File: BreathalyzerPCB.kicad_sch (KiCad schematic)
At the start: 12 parts, among them SW101 SW_SPST, U101 MAX6105, U102 ABX00030, U103 SEN-08880

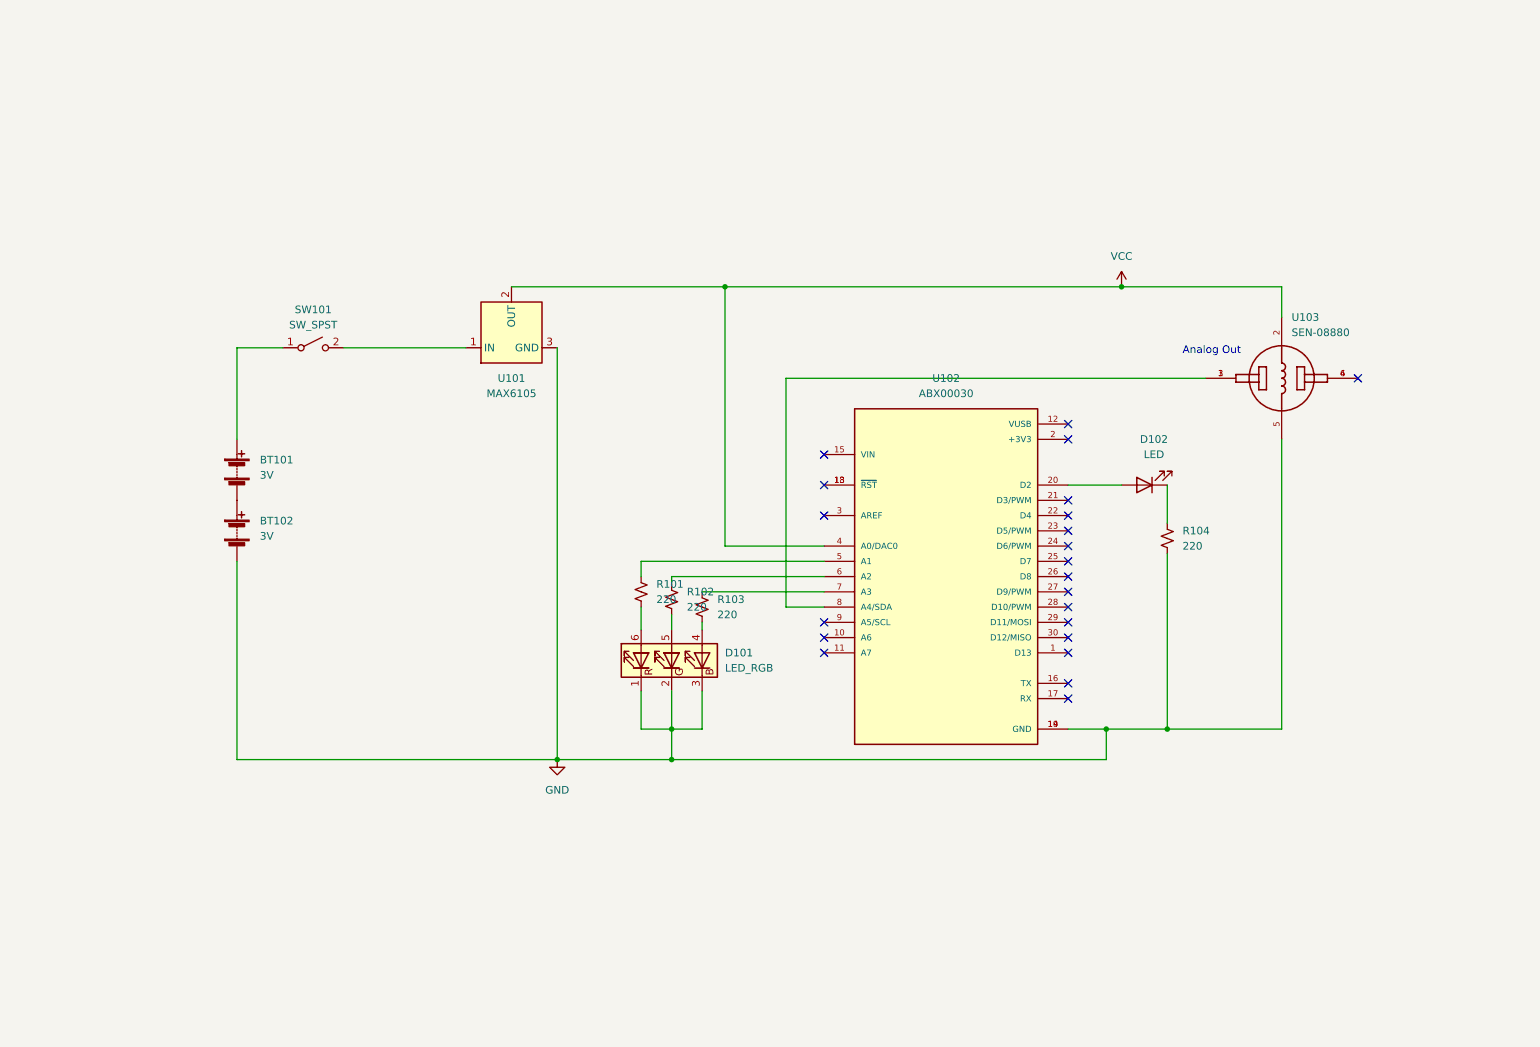
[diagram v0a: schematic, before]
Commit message: v2.1.0
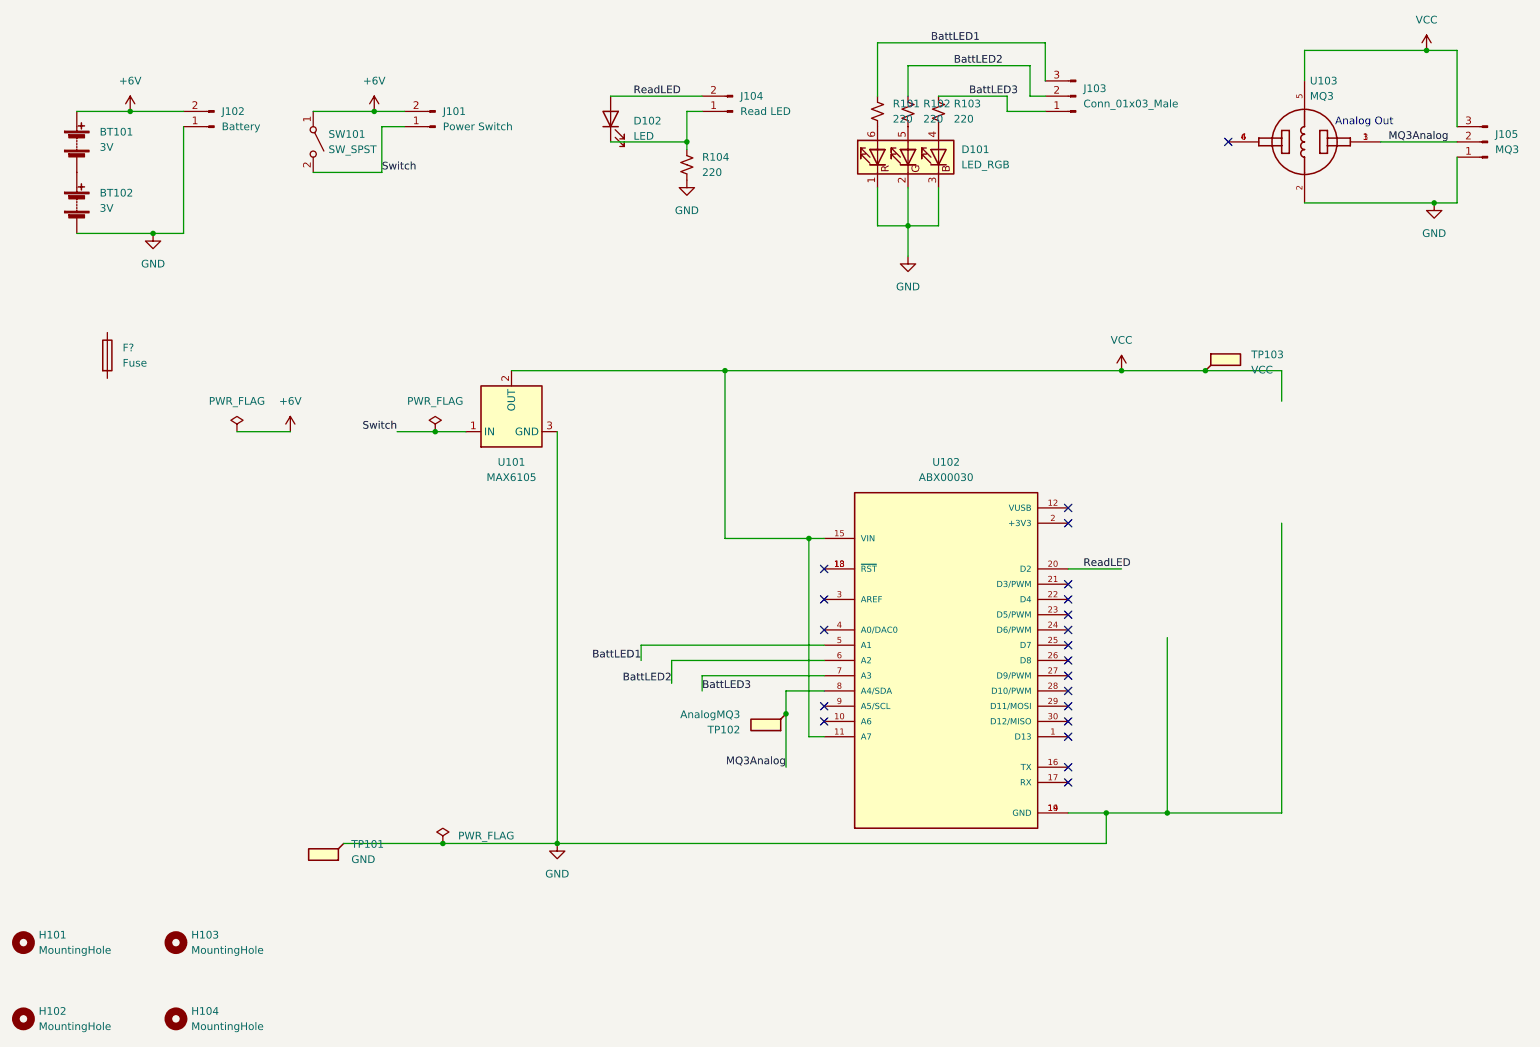
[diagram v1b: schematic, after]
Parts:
- added F?: Fuse, symbol Device:Fuse
- added H101, H102, H103, H104: MountingHole, MountingHole:MountingHole_3.2mm_M3, symbol Mechanical:MountingHole
- added J101: Power Switch, Connector_PinHeader_2.54mm:PinHeader_1x02_P2.54mm_Vertical, symbol Connector:Conn_01x02_Male
- added J102: Battery, Connector_PinHeader_2.54mm:PinHeader_1x02_P2.54mm_Vertical, symbol Connector:Conn_01x02_Male
- added J103: Conn_01x03_Male, Connector_PinHeader_2.54mm:PinHeader_1x03_P2.54mm_Vertical, symbol Connector:Conn_01x03_Male
- added J104: Read LED, Connector_PinHeader_2.54mm:PinHeader_1x02_P2.54mm_Vertical, symbol Connector:Conn_01x02_Male
- added J105: MQ3, Connector_PinHeader_2.54mm:PinHeader_1x03_P2.54mm_Vertical, symbol Connector:Conn_01x03_Male
- added TP101: GND, TestPoint:TestPoint_Pad_D4.0mm, symbol Connector:TestPoint_Flag
- added TP102: AnalogMQ3, TestPoint:TestPoint_Pad_D4.0mm, symbol Connector:TestPoint_Flag
- added TP103: VCC, TestPoint:TestPoint_Pad_D4.0mm, symbol Connector:TestPoint_Flag
- R101, R102, R103, R104: footprint (none) -> Resistor_THT:R_Axial_DIN0309_L9.0mm_D3.2mm_P12.70mm_Horizontal
- U102: footprint MODULE_ABX00030 -> Connector_PinSocket_2.54mm:PinSocket_2x14_P2.54mm_Vertical
- U103: value SEN-08880 -> MQ3
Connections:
- net GND: now also U103.2, J102.1 (Pin_1), J105.1 (Pin_1), TP101.1; no longer U103.5
- net VCC: now also U102.11 (A7), U102.15 (VIN), U103.5, J105.3 (Pin_3), TP103.1; no longer U102.4 (A0/DAC0), U103.2
- net at D102.1 (K), R104.1: now also J104.1 (Pin_1)
- net ReadLED: now reaches D102.2 (A), U102.20 (D2)
- net ReadLED: now also J104.2 (Pin_2)
- net Switch: now reaches SW101.2 (B), U101.1 (IN)
- net Switch: now also J101.1 (Pin_1)
- net +6V: now reaches BT101.1 (+), SW101.1 (A)
- net +6V: now also J101.2 (Pin_2), J102.2 (Pin_2)
- net BattLED1: now reaches R101.1, U102.5 (A1)
- net BattLED1: now also J103.3 (Pin_3)
- net BattLED2: now reaches R102.1, U102.6 (A2)
- net BattLED2: now also J103.2 (Pin_2)
- net BattLED3: now reaches R103.1, U102.7 (A3)
- net BattLED3: now also J103.1 (Pin_1)
- net MQ3Analog: now reaches U102.8 (A4/SDA), U103.1, U103.3
- net MQ3Analog: now also J105.2 (Pin_2), TP102.1
- no-connect marks 22 -> 21
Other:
- moved on the sheet: BT102, D101, D102, R101, R102, R103, R104, U101, U102, U103
